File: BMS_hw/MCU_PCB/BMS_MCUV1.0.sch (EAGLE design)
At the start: 52 parts, among them IC2 SST25VF020B804ISA, J1 22-27-2051-05, J2 22-27-2051-05, J3 22-27-2041-04, J4 22-27-2051-05, U1 NCP1117LP-PG, U2 NCP1117LP-PG, X1 87758-2016

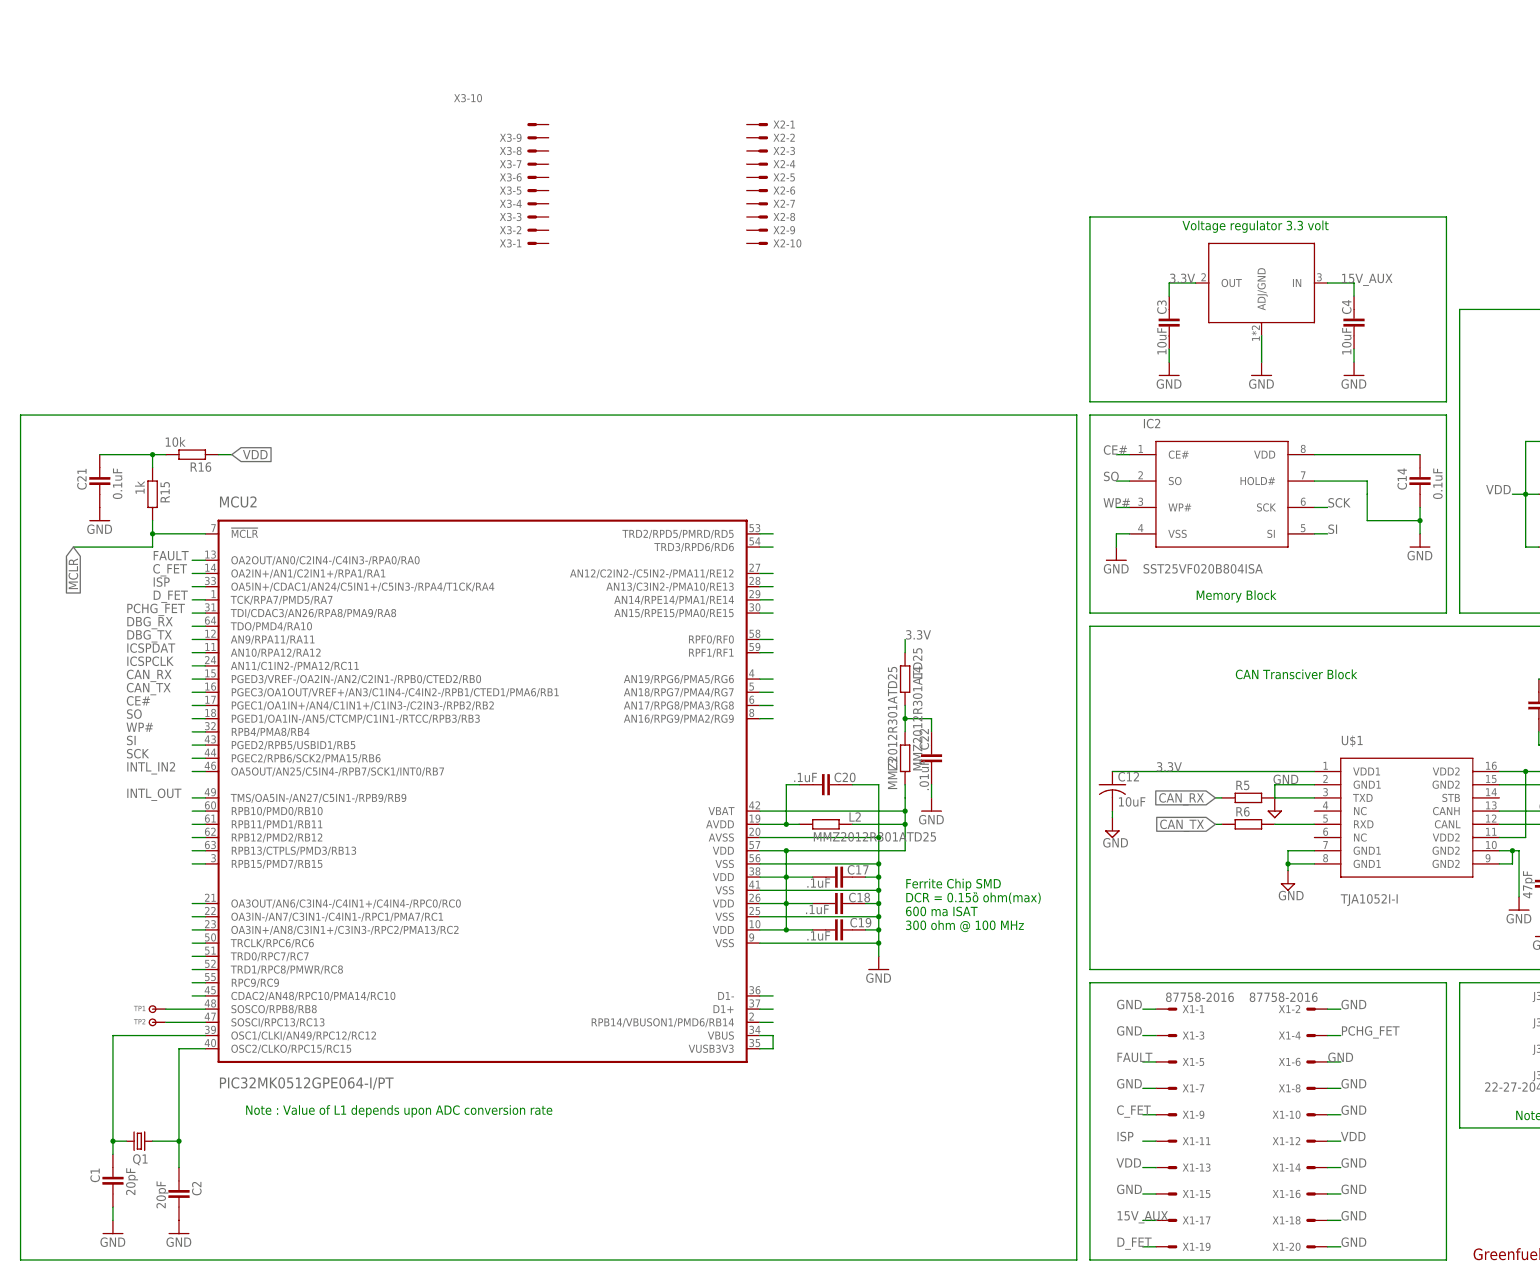
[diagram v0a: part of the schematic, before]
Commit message: hjhk
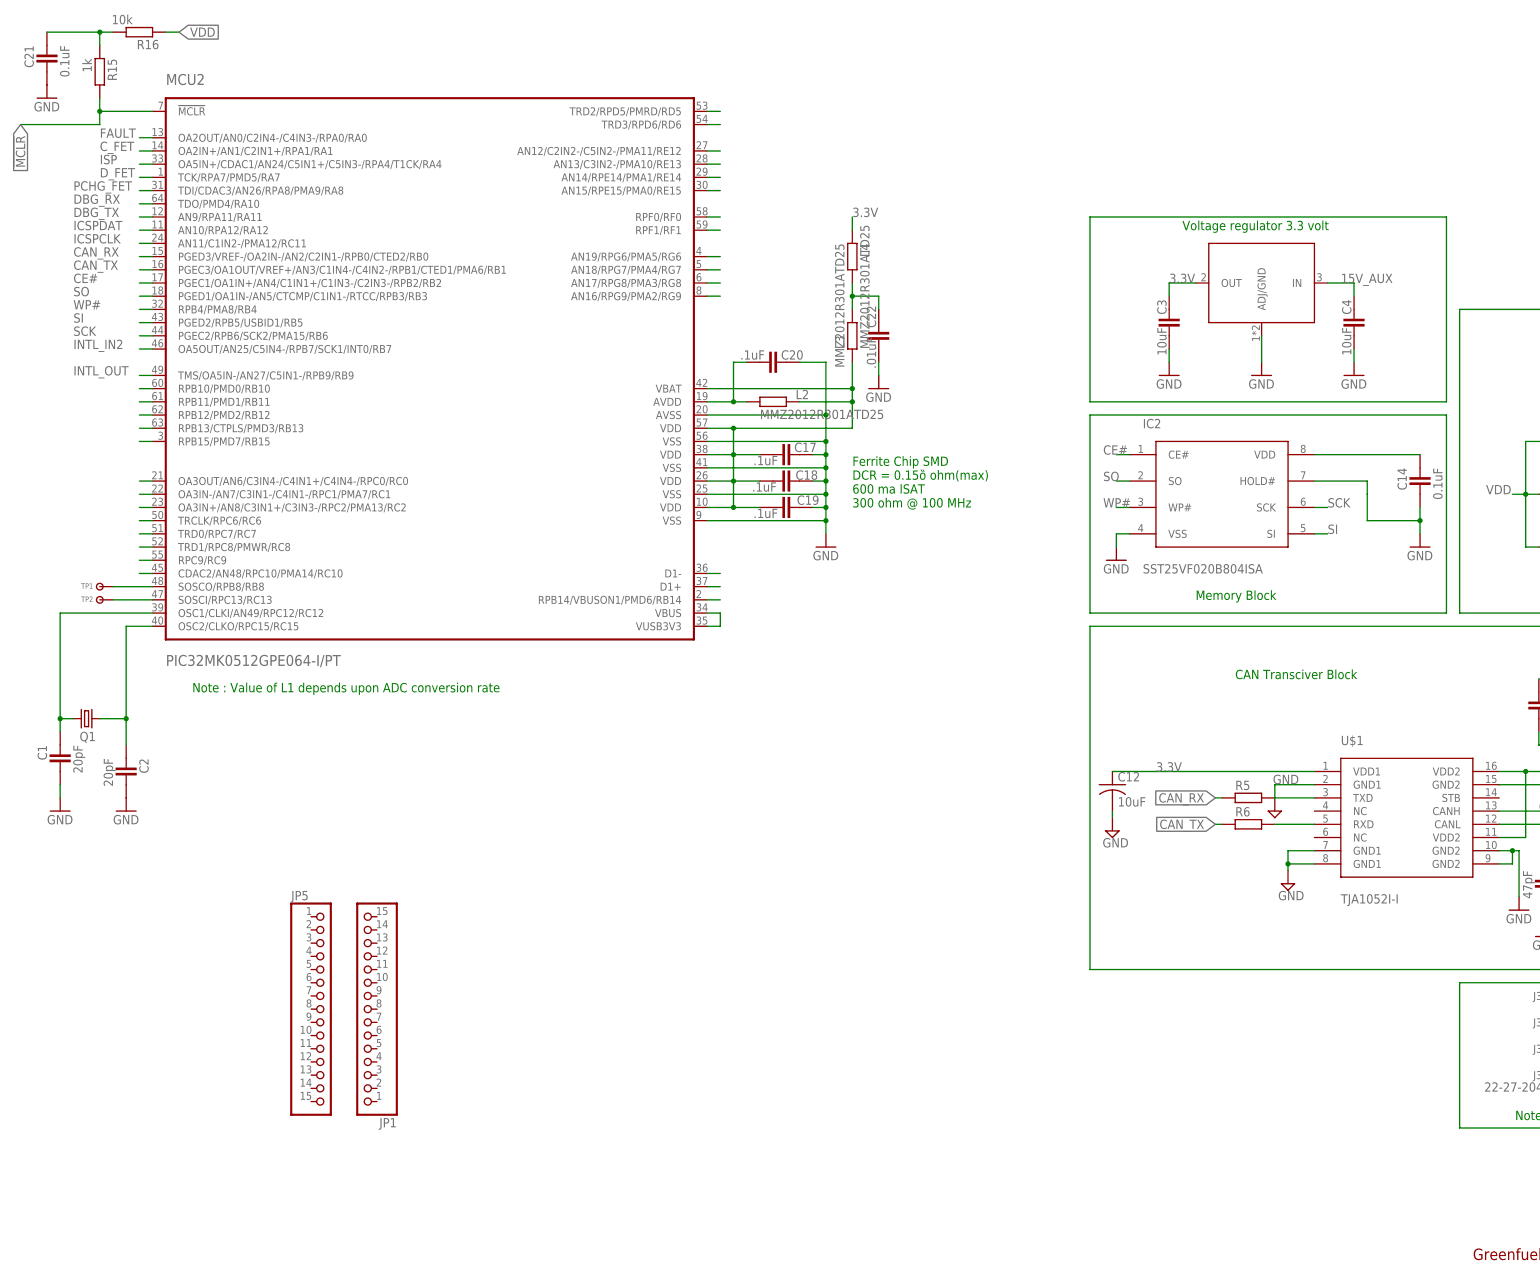
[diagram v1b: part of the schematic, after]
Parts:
- removed X1: 87758-2016, con-molex:87758-2016
- removed X2, X3: (no value), con-molex:KK-156-10
- added JP1, JP5: (no value), GreenFuel:PINHD-1X15
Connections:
- net 15V_AUX: no longer X1-17.S
- net C_FET: no longer X1-9.S
- net D_FET: no longer X1-19.S
- net FAULT: no longer X1-5.S
- net GND: no longer U$1.GND1, X1-1.S, X1-10.S, X1-14.S, X1-15.S, X1-16.S, X1-18.S, X1-2.S, X1-20.S, X1-3.S, X1-6.S, X1-7.S, X1-8.S
- net ISP: no longer X1-11.S
- net N$7: now also U$1.GND1
- net PCHG_FET: no longer X1-4.S
- net VDD: no longer X1-12.S, X1-13.S
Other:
- moved on the sheet: C1, C17, C18, C19, C2, C20, C21, C22, L2, L3, L4, MCU2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

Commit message: asdasd
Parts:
- C1, C2, C21: device ipc-7351-capacitor:CAPACITOR_0603 -> ipc-7351-capacitor:CAPACITOR_0402
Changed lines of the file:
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@@
 <parts>
 <part name="Q1" library="adafruit" deviceset="CRYSTAL" device="CTS406"/>
-<part name="C1" library="ipc-7351-capacitor" deviceset="CAPACITOR_" device="0603" value="20pF"/>
-<part name="C2" library="ipc-7351-capacitor" deviceset="CAPACITOR_" device="0603" value="20pF"/>
+<part name="C1" library="ipc-7351-capacitor" deviceset="CAPACITOR_" device="0402" value="20pF"/>
+<part name="C2" library="ipc-7351-capacitor" deviceset="CAPACITOR_" device="0402" value="20pF"/>
 <part name="GND1" library="supply1" library_urn="urn:adsk.eagle:library:371" deviceset="GND" device=""/>
 <part name="GND2" library="supply1" library_urn="urn:adsk.eagle:library:371" deviceset="GND" device=""/>
@@
 <part name="R15" library="ipc-7351-resistor" deviceset="RESISTOR_" device="0603" value="1k"/>
 <part name="R16" library="ipc-7351-resistor" deviceset="RESISTOR_" device="0603" value="10k"/>
-<part name="C21" library="ipc-7351-capacitor" deviceset="CAPACITOR_" device="0603" value="0.1uF"/>
+<part name="C21" library="ipc-7351-capacitor" deviceset="CAPACITOR_" device="0402" value="0.1uF"/>
 <part name="GND22" library="supply1" library_urn="urn:adsk.eagle:library:371" deviceset="GND" device=""/>
 <part name="L3" library="ipc-7351-resistor" deviceset="RESISTOR_" device="0805" value="MMZ2012R301ATD25"/>

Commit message: brd layout and sch updated!
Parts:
- C10, C13, C7, C9: device ipc-7351-capacitor:CAPACITOR_0805 -> ipc-7351-capacitor:CAPACITOR_0402
- C11, C12, C8: device adafruit:C-USC0805 -> ipc-7351-capacitor:CAPACITOR_0402
- C14, C17, C18, C19, C20, C22, C3, C4: device ipc-7351-capacitor:CAPACITOR_0603 -> ipc-7351-capacitor:CAPACITOR_0402
- Q1: value (none) -> CRYSTALS-GND-LID-IQXC-42; device adafruit:CRYSTALCTS406 -> IQD-Frequency-Products:CRYSTALS-GND-LID-IQXC-42
- R10, R11, R12, R13, R14, R3, R4, R5, R6, R7, R8, R9: device ipc-7351-resistor:RESISTOR_0805 -> ipc-7351-resistor:RESISTOR_0402
- R15, R16: device ipc-7351-resistor:RESISTOR_0603 -> ipc-7351-resistor:RESISTOR_0402
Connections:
- new net N$3: C12.1, U$1.VDD1
- net 3.3V: no longer C12.1, U$1.VDD1
- net GND: now also Q1.2, Q1.4
- net N$1: now also Q1.3; no longer Q1.2
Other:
- moved on the sheet: C1, C11, C12, C2, C8
